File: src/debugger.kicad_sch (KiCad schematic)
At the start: 29 parts, among them J2 USB_C_Receptacle_USB2.0_14P, U7 RP2040, U8 W25Q128JVS, U9 NCP1117-1.5_SOT223, Y1 ABM8-272-T3

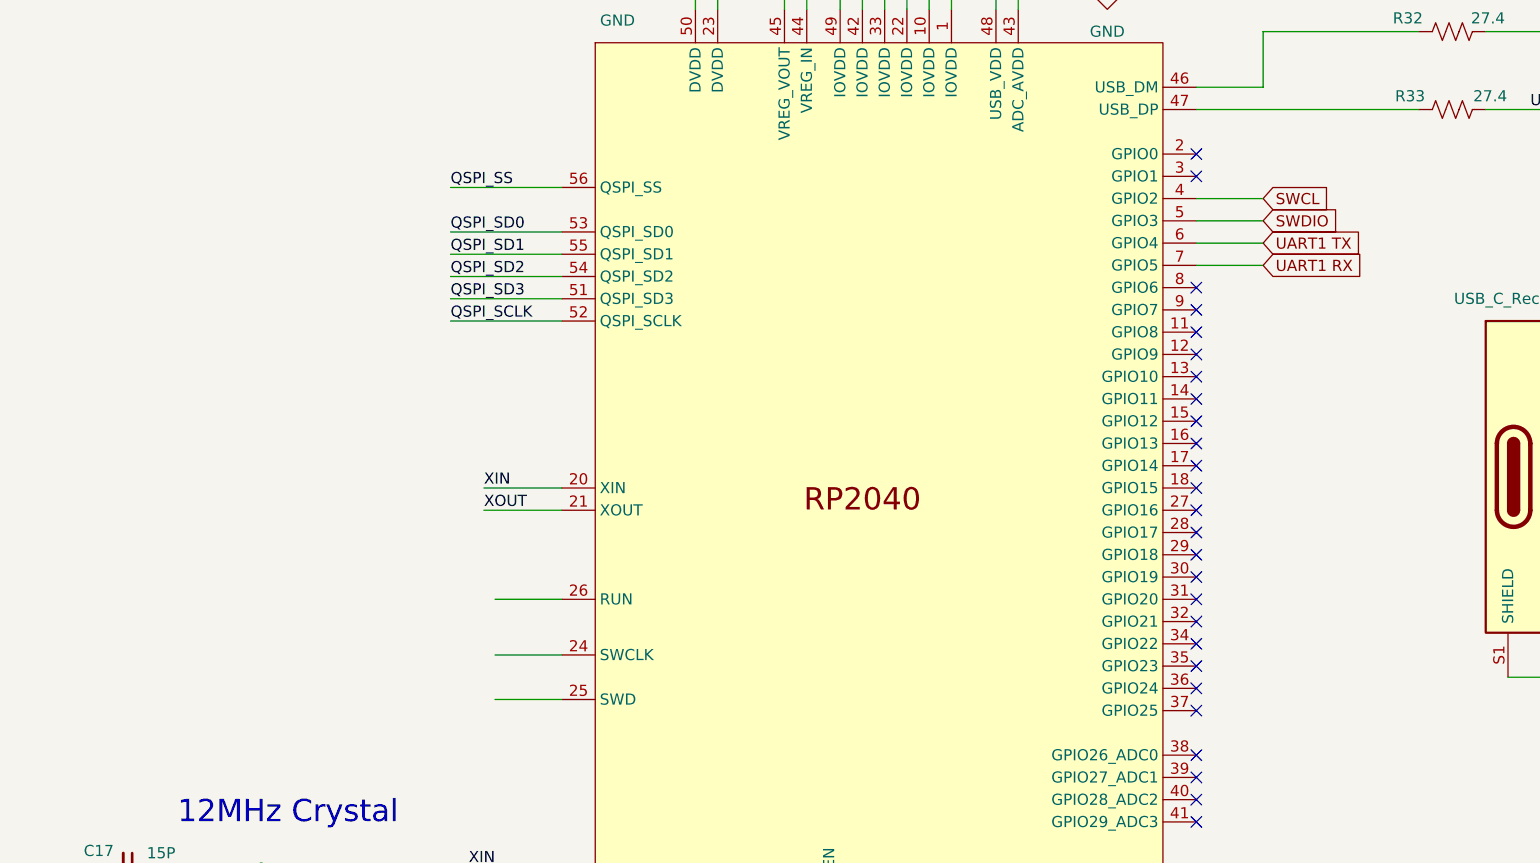
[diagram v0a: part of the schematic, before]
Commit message: revisão da RP2040
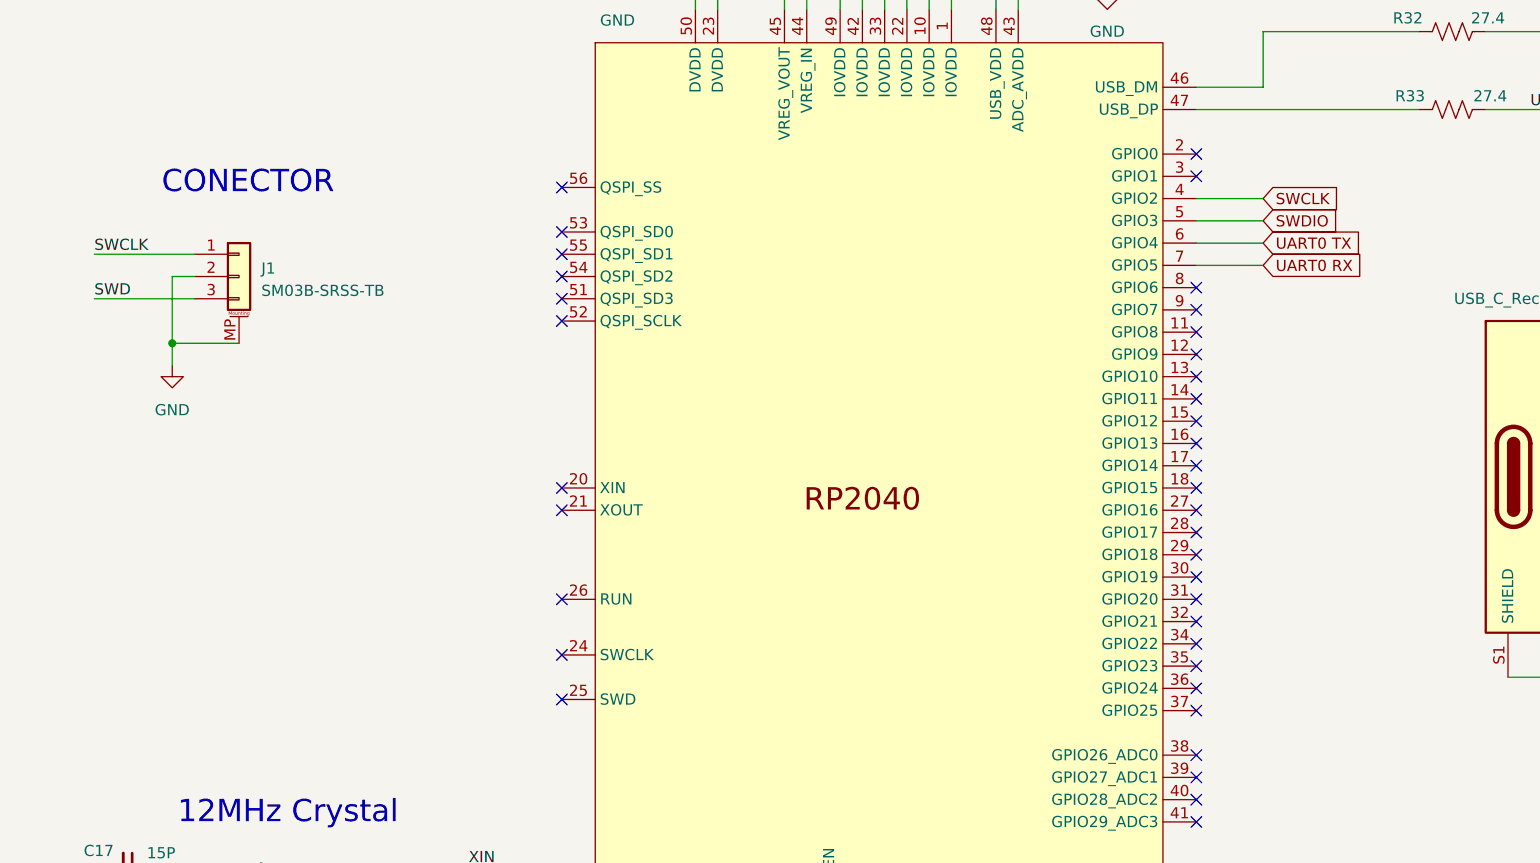
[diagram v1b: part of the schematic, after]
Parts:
- added J1: SM03B-SRSS-TB, Connector_JST:JST_SH_SM03B-SRSS-TB_1x03-1MP_P1.00mm_Horizontal, symbol Connector_Generic_MountingPin:Conn_01x03_MountingPin
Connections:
- net GND: now also J1.2 (Pin_2), J1.MP (MountPin)
- net QSPI_SCLK: no longer U7.52 (QSPI_SCLK)
- net QSPI_SD0: no longer U7.53 (QSPI_SD0)
- net QSPI_SD1: no longer U7.55 (QSPI_SD1)
- net QSPI_SD2: no longer U7.54 (QSPI_SD2)
- net QSPI_SD3: no longer U7.51 (QSPI_SD3)
- net QSPI_SS: no longer U7.56 (QSPI_SS)
- net XIN: no longer U7.20 (XIN)
- net XOUT: no longer U7.21 (XOUT)
- net SWCL renamed SWCLK
- net SWCLK: now also J1.1 (Pin_1)
- net UART1 RX renamed UART0 RX
- net UART1 TX renamed UART0 TX
- new net SWD: J1.3 (Pin_3)
- no-connect marks 26 -> 37
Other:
- note added: "CONECTOR"

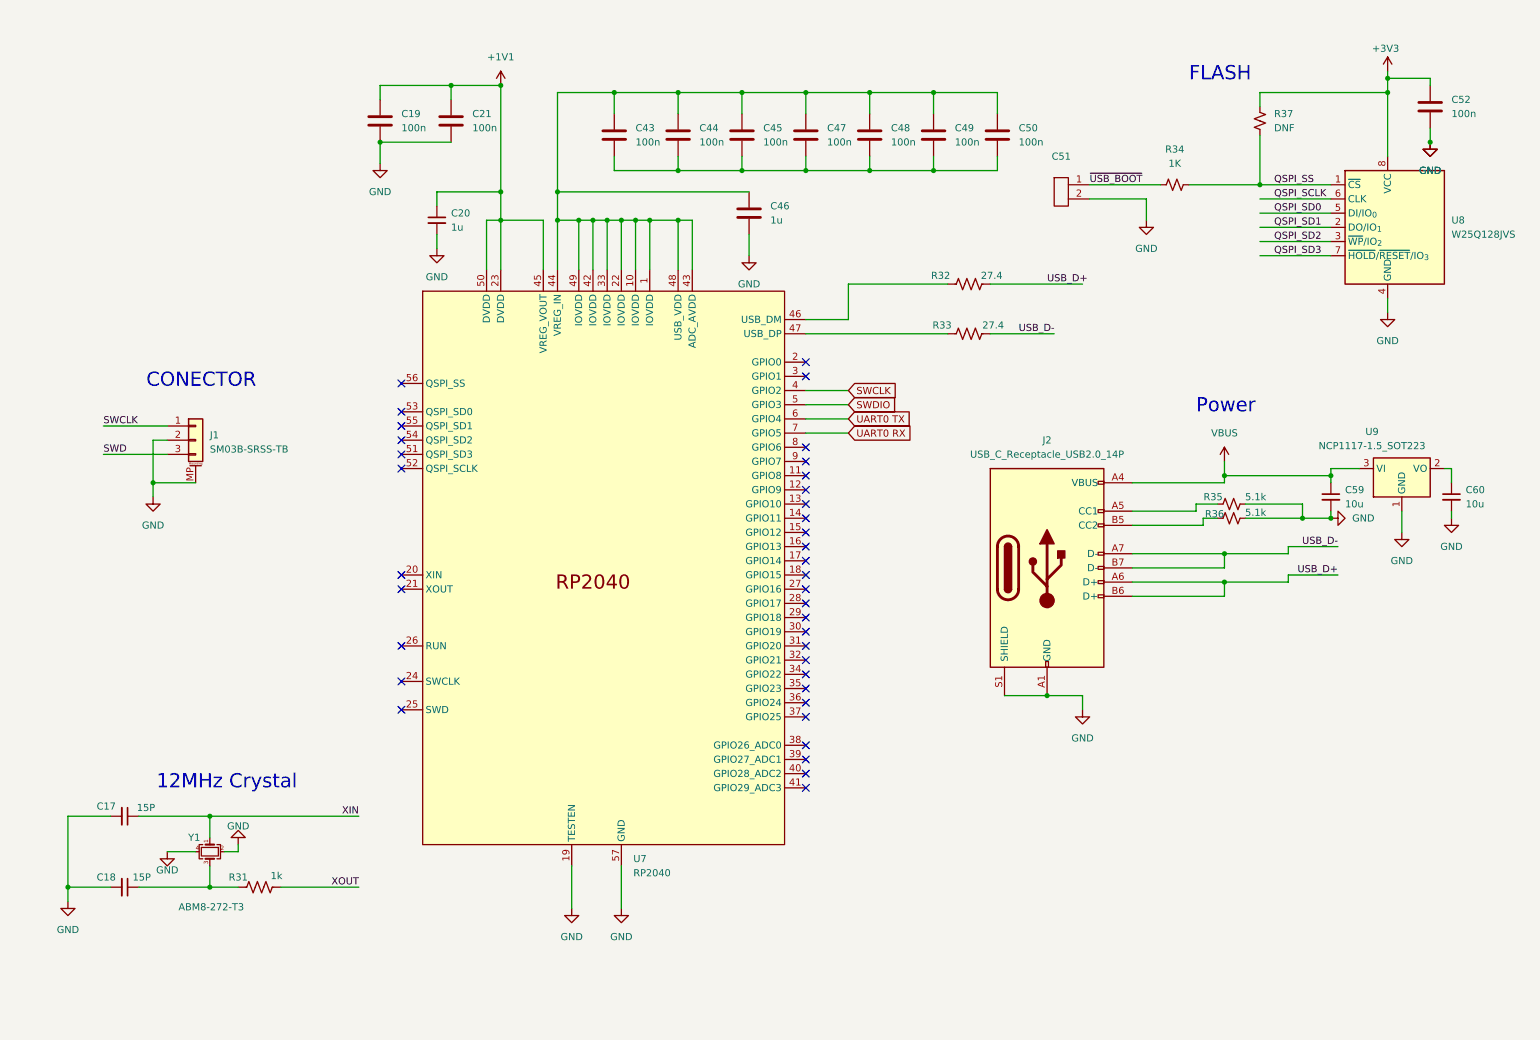
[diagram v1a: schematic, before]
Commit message: FEAT: adicionando footprints
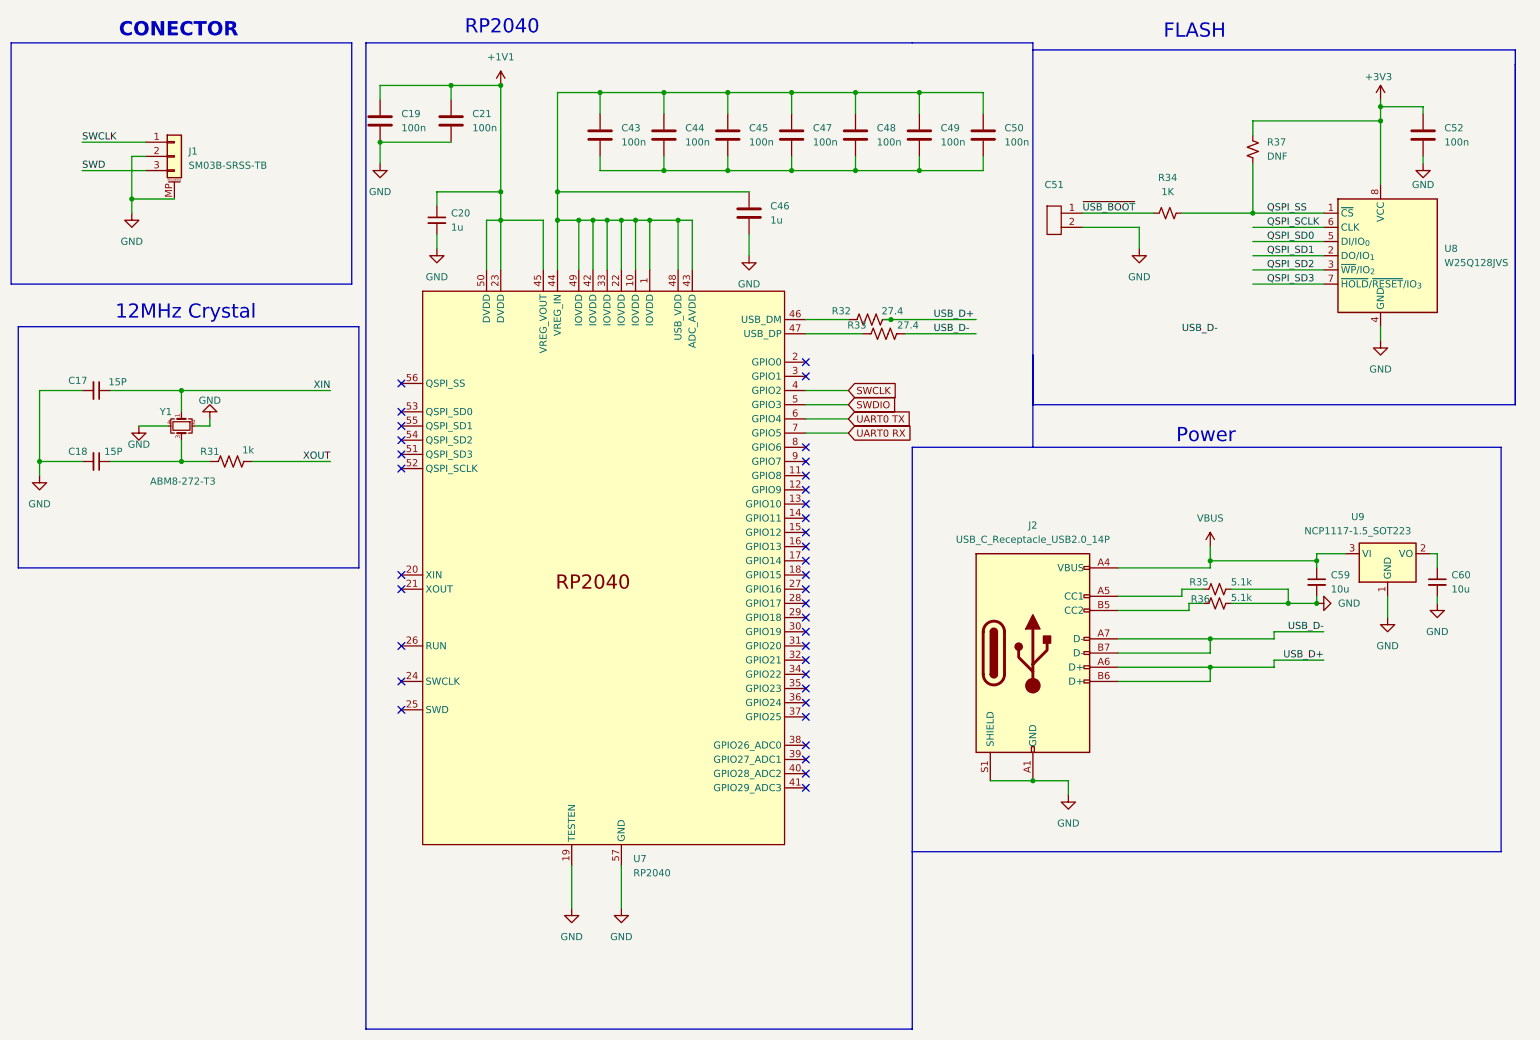
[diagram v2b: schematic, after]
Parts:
- J2: footprint (none) -> Connector_USB:USB_C_Receptacle_GCT_USB4105-xx-A_16P_TopMnt_Horizontal
- U7: footprint (none) -> componentes_personalizados:RP2040
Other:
- note added: "RP2040"
- moved on the sheet: C17, C18, C43, C44, C45, C47, C48, C49, C50, C51, C52, C59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
